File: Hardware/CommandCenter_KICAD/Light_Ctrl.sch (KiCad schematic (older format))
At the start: 49 parts

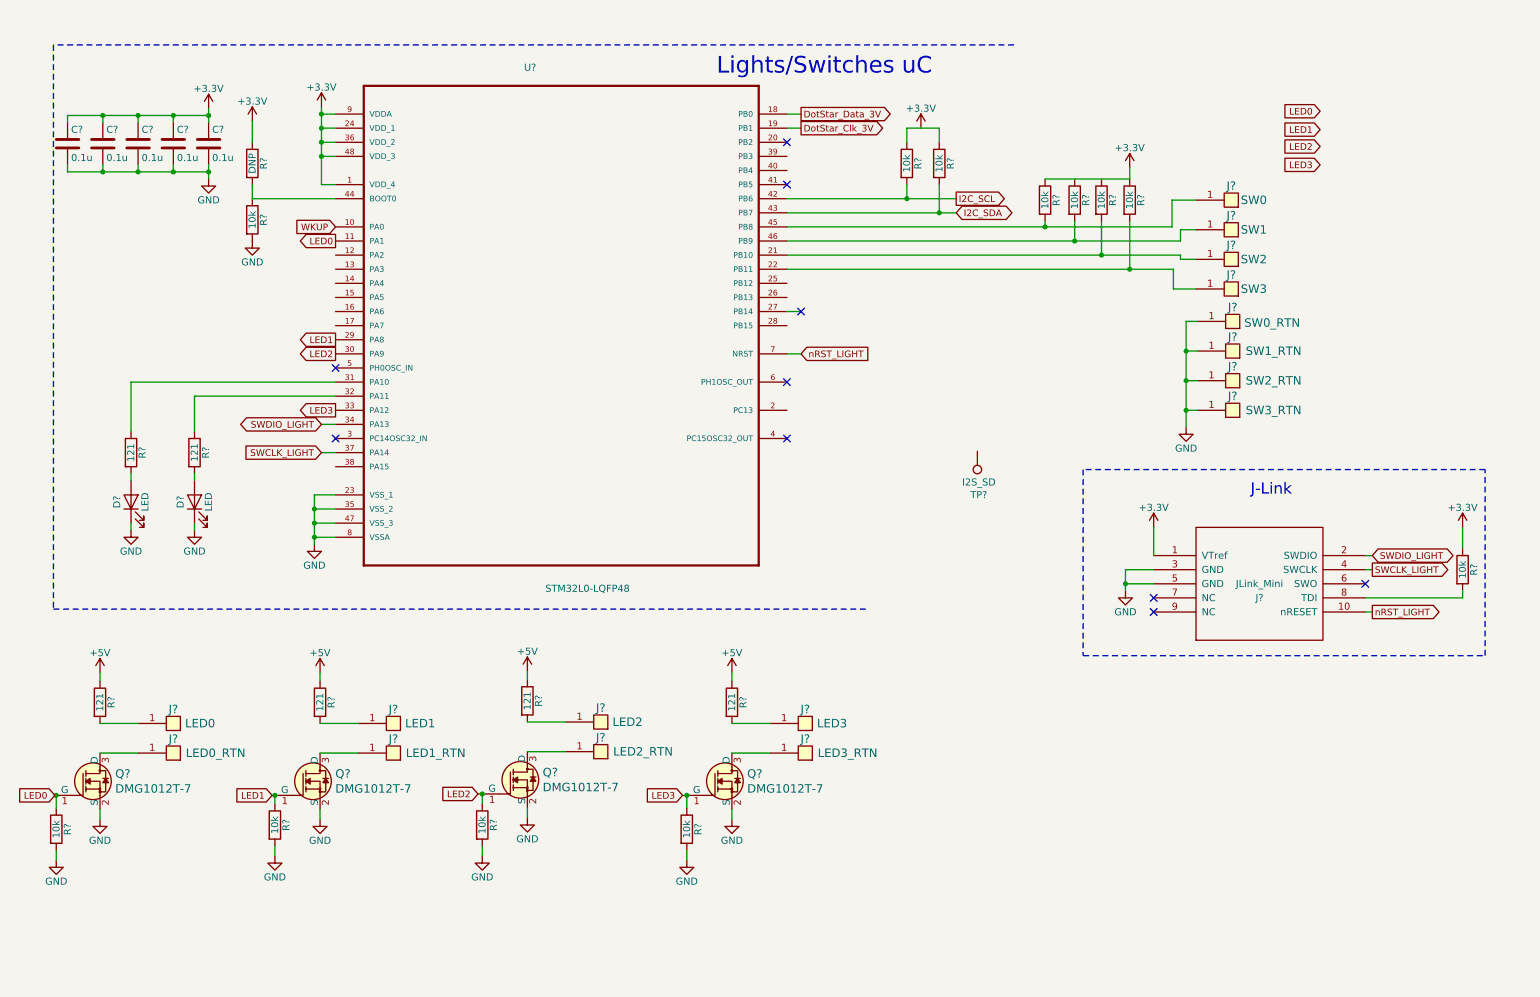
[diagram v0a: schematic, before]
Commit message: Layout started
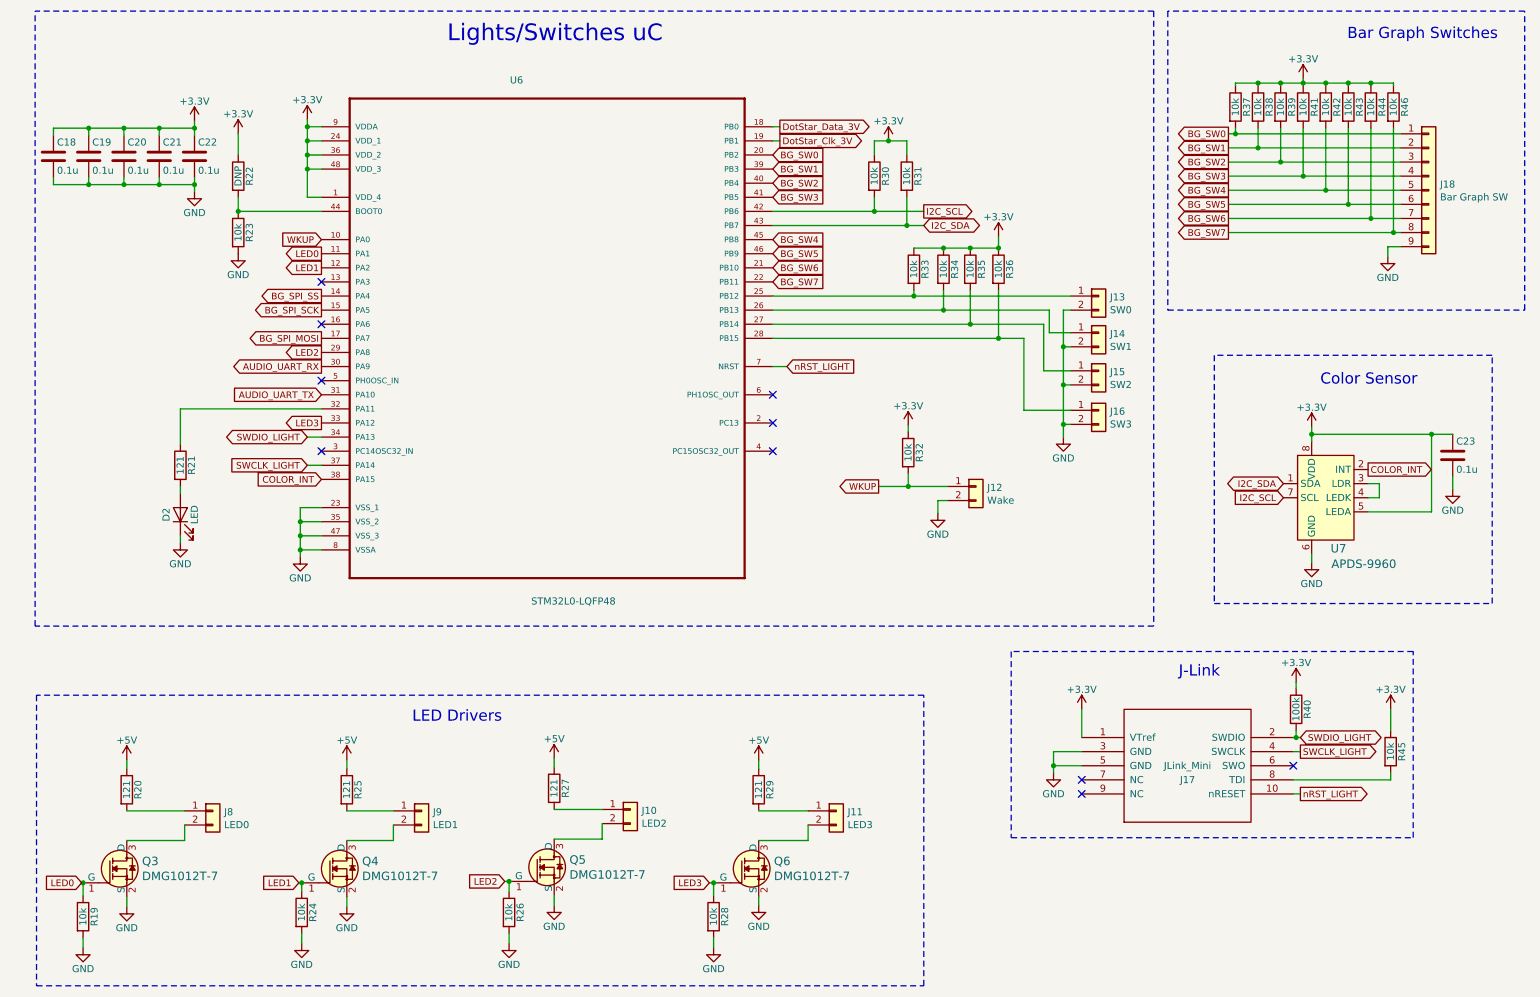
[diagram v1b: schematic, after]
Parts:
- removed D?: LED, LEDs:LED_0603_HandSoldering, symbol Device:LED
- removed J?: SW0, NFC_Toy_Lib:Pad_SMD_Small, symbol Pad:Pad
- removed J?: SW1, NFC_Toy_Lib:Pad_SMD_Small, symbol Pad:Pad
- removed J?: SW2, NFC_Toy_Lib:Pad_SMD_Small, symbol Pad:Pad
- removed J?: SW3, NFC_Toy_Lib:Pad_SMD_Small, symbol Pad:Pad
- removed J?: SW0_RTN, NFC_Toy_Lib:Pad_SMD_Small, symbol Pad:Pad
- removed J?: SW1_RTN, NFC_Toy_Lib:Pad_SMD_Small, symbol Pad:Pad
- removed J?: SW2_RTN, NFC_Toy_Lib:Pad_SMD_Small, symbol Pad:Pad
- removed J?: SW3_RTN, NFC_Toy_Lib:Pad_SMD_Small, symbol Pad:Pad
- removed J?: LED0, NFC_Toy_Lib:Pad_SMD_Small, symbol Pad:Pad
- removed J?: LED0_RTN, NFC_Toy_Lib:Pad_SMD_Small, symbol Pad:Pad
- removed J?: LED1, NFC_Toy_Lib:Pad_SMD_Small, symbol Pad:Pad
- removed J?: LED1_RTN, NFC_Toy_Lib:Pad_SMD_Small, symbol Pad:Pad
- removed J?: LED2, NFC_Toy_Lib:Pad_SMD_Small, symbol Pad:Pad
- removed J?: LED2_RTN, NFC_Toy_Lib:Pad_SMD_Small, symbol Pad:Pad
- removed J?: LED3, NFC_Toy_Lib:Pad_SMD_Small, symbol Pad:Pad
- removed J?: LED3_RTN, NFC_Toy_Lib:Pad_SMD_Small, symbol Pad:Pad
- removed R?: 121, Resistors_SMD:R_0603_HandSoldering, symbol Device:R
- removed TP?: I2S_SD, symbol Connector:TestPoint
- added C23: 0.1u, Capacitor_SMD:C_0603_1608Metric_Pad1.05x0.95mm_HandSolder, symbol Device:C
- added J10: LED2, Connector_PinHeader_2.54mm:PinHeader_1x02_P2.54mm_Vertical, symbol Connector_Generic:Conn_01x02
- added J11: LED3, Connector_PinHeader_2.54mm:PinHeader_1x02_P2.54mm_Vertical, symbol Connector_Generic:Conn_01x02
- added J12: Wake, Connector_PinHeader_2.54mm:PinHeader_1x02_P2.54mm_Vertical, symbol Connector_Generic:Conn_01x02
- added J13: SW0, Connector_PinHeader_2.54mm:PinHeader_1x02_P2.54mm_Vertical, symbol Connector_Generic:Conn_01x02
- added J14: SW1, Connector_PinHeader_2.54mm:PinHeader_1x02_P2.54mm_Vertical, symbol Connector_Generic:Conn_01x02
- added J15: SW2, Connector_PinHeader_2.54mm:PinHeader_1x02_P2.54mm_Vertical, symbol Connector_Generic:Conn_01x02
- added J16: SW3, Connector_PinHeader_2.54mm:PinHeader_1x02_P2.54mm_Vertical, symbol Connector_Generic:Conn_01x02
- added J18: Bar Graph SW, Connector_PinHeader_2.54mm:PinHeader_1x09_P2.54mm_Vertical, symbol Connector_Generic:Conn_01x09
- added J8: LED0, Connector_PinHeader_2.54mm:PinHeader_1x02_P2.54mm_Vertical, symbol Connector_Generic:Conn_01x02
- added J9: LED1, Connector_PinHeader_2.54mm:PinHeader_1x02_P2.54mm_Vertical, symbol Connector_Generic:Conn_01x02
- added R32, R37, R38, R39, R41, R42, R43, R44, R46: 10k, Resistor_SMD:R_0603_1608Metric_Pad1.05x0.95mm_HandSolder, symbol Device:R
- added R40: 100k, Resistor_SMD:R_0603_1608Metric_Pad1.05x0.95mm_HandSolder, symbol Device:R
- added U7: APDS-9960, digikey-footprints:Ambient_Prox_APDS-9960, symbol dk_Optical-Sensors-Ambient-Light-IR-UV-Sensors:APDS-9960
- C18, C19, C20, C21, C22: renamed from C?; footprint Capacitors_SMD:C_0402 -> Capacitor_SMD:C_0603_1608Metric_Pad1.05x0.95mm_HandSolder
- D2: renamed from D?; footprint LEDs:LED_0603_HandSoldering -> LED_SMD:LED_0603_1608Metric_Pad1.05x0.95mm_HandSolder
- J17: renamed from J?; footprint Socket_Strips:Socket_Strip_Straight_2x05_Pitch2.54mm_SMD -> CommandCenter:JLink_Mini_0p05
- R19, R20, R21, R22, R23, R24, R25, R26, R27, R28, R29, R30, R31, R33, R34, R35, R36, R45: renamed from R?; footprint Resistors_SMD:R_0603_HandSoldering -> Resistor_SMD:R_0603_1608Metric_Pad1.05x0.95mm_HandSolder
- U6: renamed from U?; footprint NFC_Toy_Lib:QFP50P900X900X160-48N -> CommandCenter:QFP50P900X900X160-48N
- gave numbers to parts that had none: 4
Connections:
- net +3V3: now also R30.1, R31.1, R34.1, R35.1, C23.1, R32.1, R37.1, R38.1, R39.1, R40.1, R41.1, U7.5 (LEDA), U7.8 (VDD)
- net GND: now also C23.2, J12.2 (Pin_2), J13.2 (Pin_2), J14.2 (Pin_2), J15.2 (Pin_2), J16.2 (Pin_2), J18.9 (Pin_9), U7.6 (GND)
- net I2C_SCL: now also U7.7 (SCL)
- net I2C_SDA: now also U7.1 (SDA)
- net LED1: now also U6.12 (PA2); no longer U6.29 (PA8)
- net LED2: now also U6.29 (PA8); no longer U6.30 (PA9)
- net SWDIO_LIGHT: now also R40.2
- net WKUP: now also J12.1 (Pin_1), R32.2
- net BG_SPI_SS: now reaches U6.14 (PA4)
- net BG_SPI_SCK: now reaches U6.15 (PA5)
- net BG_SPI_MOSI: now reaches U6.17 (PA7)
- net BG_SW0: now reaches U6.20 (PB2)
- net BG_SW0: now also J18.1 (Pin_1), R37.2
- net at R35.2: now also U6.27 (PB14), J15.1 (Pin_1); no longer U6.21 (PB10)
- net at R36.2: now also U6.28 (PB15), J16.1 (Pin_1); no longer U6.22 (PB11)
- net at U6.25 (PB12): now also R33.2, J13.1 (Pin_1)
- net at U6.26 (PB13): now also R34.2, J14.1 (Pin_1)
- net AUDIO_UART_TX: now reaches U6.31 (PA10)
- net COLOR_INT: now reaches U6.38 (PA15)
- net COLOR_INT: now also U7.2 (INT)
- net BG_SW1: now reaches U6.39 (PB3)
- net BG_SW1: now also J18.2 (Pin_2), R38.2
- net BG_SW2: now reaches U6.40 (PB4)
- net BG_SW2: now also J18.3 (Pin_3), R39.2
- net BG_SW3: now reaches U6.41 (PB5)
- net BG_SW3: now also J18.4 (Pin_4), R41.2
- net BG_SW4: now reaches U6.45 (PB8)
- net BG_SW4: now also J18.5 (Pin_5), R42.2; no longer R33.2
- net BG_SW5: now reaches U6.46 (PB9)
- net BG_SW5: now also J18.6 (Pin_6), R43.2; no longer R34.2
- net at Q3.3 (D): now also J8.2 (Pin_2)
- net at R20.2: now also J8.1 (Pin_1)
- net at Q4.3 (D): now also J9.2 (Pin_2)
- net at R25.2: now also J9.1 (Pin_1)
- net at Q5.3 (D): now also J10.2 (Pin_2)
- net at R27.2: now also J10.1 (Pin_1)
- net at Q6.3 (D): now also J11.2 (Pin_2)
- net at R29.2: now also J11.1 (Pin_1)
- new net: U7.3 (LDR), U7.4 (LEDK)
- new net: R42.1, R43.1, R44.1, R46.1
- new net AUDIO_UART_RX: U6.30 (PA9)
- new net BG_SW6: J18.7 (Pin_7), R44.2, U6.21 (PB10)
- new net BG_SW7: J18.8 (Pin_8), R46.2, U6.22 (PB11)
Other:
- note added: "Bar Graph Switches"
- note added: "Color Sensor"
- note added: "LED Drivers"
- moved on the sheet: C18, C19, C20, C21, C22, D2, J17, Q3, Q4, Q5, Q6, R19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
